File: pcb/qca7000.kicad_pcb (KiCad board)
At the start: 2 copper layers, 84.7 x 89.1 mm, 209 parts, among them J1 Conn_01x04_Pin, J10 CP/PE, J11 spare, J2 Conn_01x08_Pin, J3 CAN, J4 DEBUG, J5 UART, J6 12V_in, J7 RF, J8 CONTACTORS, J9 Temps, Q1 BC846, Q2 NCV8402xST, Q3 NCV8402xST, U1 25Q16, U2 SN65HVD234, U3 STM32F103RETx, U4 TPS54302, U5 AMS1117-3.3, U6 AMS1117-3.3, U7 74HCT04, Y1 25MHz, Y2 8MHz

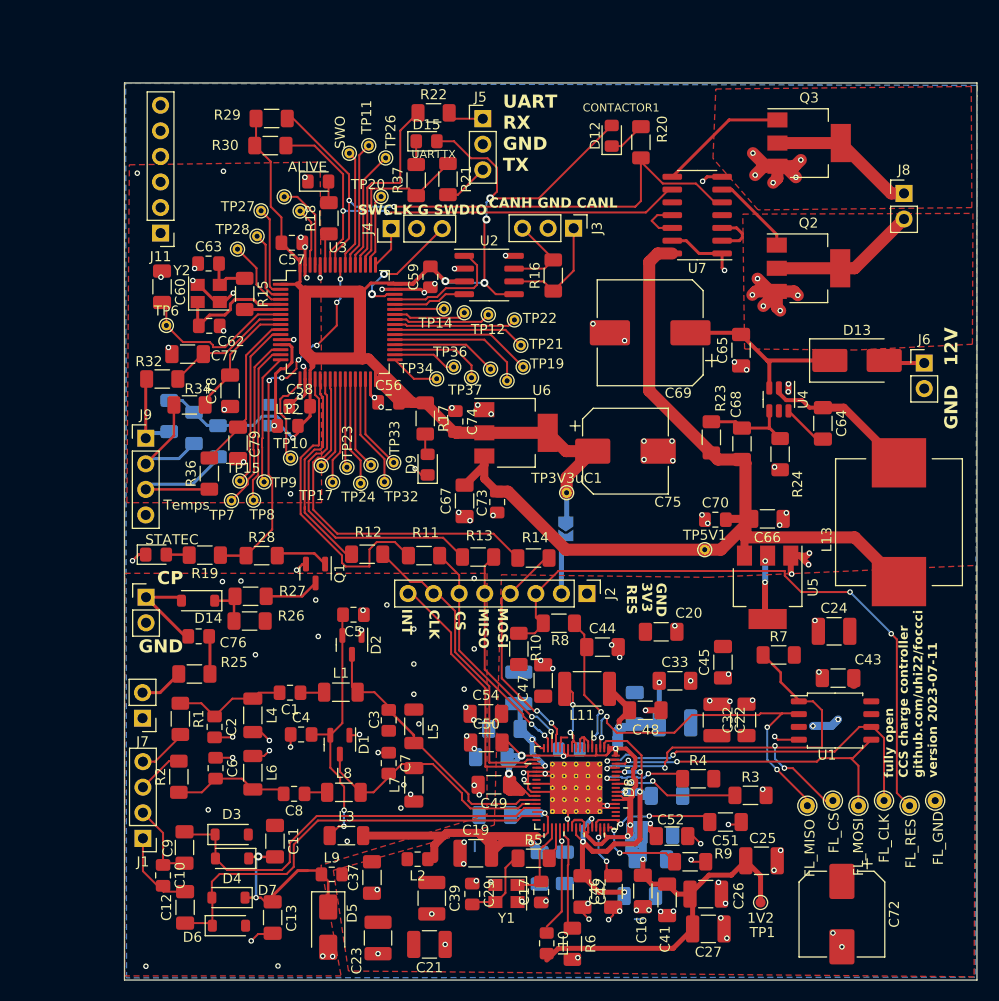
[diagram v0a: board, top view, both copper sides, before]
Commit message: fix: divider on the stepdown. fix: non-inverted contactor drivers. fix: part number of 8MHz. add: mounting holes and spare grid. add: LIM HVDC input. docu: todo list
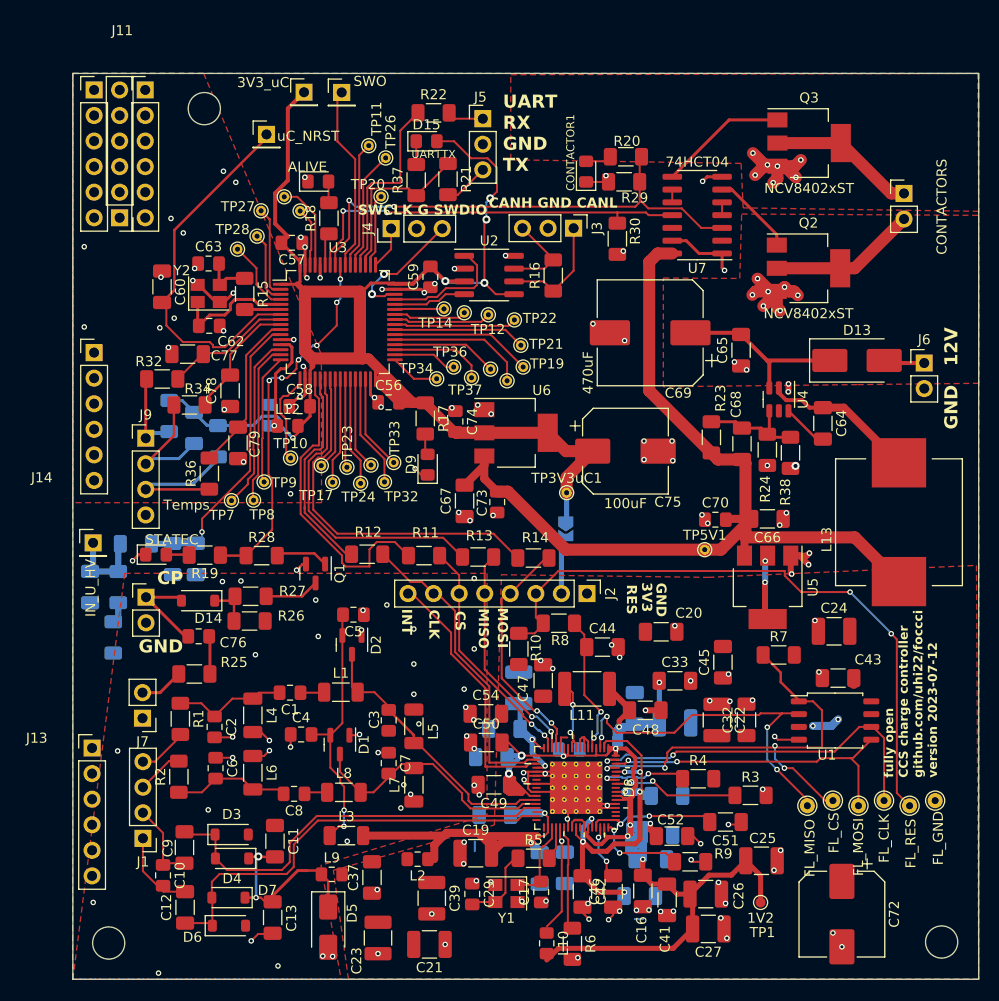
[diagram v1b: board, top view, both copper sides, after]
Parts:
- removed TP15: ~, TestPoint:TestPoint_THTPad_D1.0mm_Drill0.5mm
- removed TP35: SWO, TestPoint:TestPoint_THTPad_D1.0mm_Drill0.5mm
- removed TP6: uC_RESET, TestPoint:TestPoint_THTPad_D1.0mm_Drill0.5mm
- added C71: 100nF, Capacitor_SMD:C_1206_3216Metric_Pad1.33x1.80mm_HandSolder, B.Cu at (117.7, 90.0)
- added C80: 100nF, Capacitor_SMD:C_1206_3216Metric_Pad1.33x1.80mm_HandSolder, B.Cu at (128.2, 87.2)
- added H1: MountingHole, MountingHole:MountingHole_3.2mm_M3, F.Cu at (129.1, 42.5)
- added H2: MountingHole, MountingHole:MountingHole_3.2mm_M3, F.Cu at (119.6, 125.4)
- added H3: MountingHole, MountingHole:MountingHole_3.2mm_M3, F.Cu at (202.3, 125.3)
- added J12: spare, Connector_PinHeader_2.54mm:PinHeader_1x06_P2.54mm_Vertical, F.Cu at (123.2, 40.6)
- added J13: spare, Connector_PinHeader_2.54mm:PinHeader_1x06_P2.54mm_Vertical, F.Cu at (117.9, 106.0)
- added J14: spare, Connector_PinHeader_2.54mm:PinHeader_1x06_P2.54mm_Vertical, F.Cu at (118.1, 66.7)
- added J15: spare, Connector_PinHeader_2.54mm:PinHeader_1x06_P2.54mm_Vertical, F.Cu at (118.1, 40.6)
- added J16: uC_NRST, Connector_PinHeader_2.54mm:PinHeader_1x01_P2.54mm_Vertical, F.Cu at (135.2, 45.1)
- added J17: 3V3_uC, Connector_PinHeader_2.54mm:PinHeader_1x01_P2.54mm_Vertical, F.Cu at (139.0, 40.9)
- added J18: SWO, Connector_PinHeader_2.54mm:PinHeader_1x01_P2.54mm_Vertical, F.Cu at (142.7, 40.9)
- added J19: IN_U_HV, Connector_PinHeader_2.54mm:PinHeader_1x01_P2.54mm_Vertical, F.Cu at (118.0, 85.6)
- added R38: 22k, Resistor_SMD:R_1206_3216Metric_Pad1.30x1.75mm_HandSolder, F.Cu at (187.3, 76.7)
- added R39: 240, Resistor_SMD:R_1206_3216Metric_Pad1.30x1.75mm_HandSolder, B.Cu at (120.5, 90.0)
- added R40: 240, Resistor_SMD:R_1206_3216Metric_Pad1.30x1.75mm_HandSolder, B.Cu at (120.0, 95.0)
- added R41: 47k, Resistor_SMD:R_1206_3216Metric_Pad1.30x1.75mm_HandSolder, B.Cu at (122.3, 85.7)
- added R42: 22k, Resistor_SMD:R_1206_3216Metric_Pad1.30x1.75mm_HandSolder, B.Cu at (125.9, 87.2)
- R23: value 10k -> 100k
- R24: value 10k -> 33k
- moved R30 35.7 mm to (170.1, 55.4), turned to 90 degrees
- moved R29 35.6 mm to (170.8, 49.8)
- moved D12 4.38 mm to (167.0, 48.8)
- moved J11 4.34 mm to (120.7, 53.3)
- moved R20 2.07 mm to (170.9, 47.3), turned to 180 degrees
- moved R24 1.34 mm to (185.0, 76.4)
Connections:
- net uC_RESET renamed uC_NRST
- D12 pad 1: Net-(D12-K) -> GND
- D12 pad 2: 3V3_uC -> Net-(D12-A)
- R20 pad 2: Net-(D12-K) -> Net-(D12-A)
- R29 pad 2: 3V3_uC -> GND
- R30 pad 1: 3V3_uC -> GND
- U3 pad 11: Net-(U3-PC3) -> ADC_U_HVDC
- U7 pad 10: unconnected-(U7-Pad10) -> Net-(U7-Pad10)
- U7 pad 11: Net-(U7-Pad11) -> CONTACTOR_CONTROL2
- U7 pad 12: Net-(U7-Pad11) -> unconnected-(U7-Pad12)
- U7 pad 2: Net-(U7-Pad2) -> unconnected-(U7-Pad2)
- U7 pad 3: Net-(U7-Pad2) -> CONTACTOR_CONTROL1
- U7 pad 4: unconnected-(U7-Pad4) -> Net-(U7-Pad4)
- U7 pad 5: CONTACTOR_CONTROL1 -> Net-(U7-Pad4)
- U7 pad 9: CONTACTOR_CONTROL2 -> Net-(U7-Pad10)
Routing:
- net ADC_U_HVDC: track 0.00 -> 29.2 mm, vias 0 -> 1
- net uC_NRST: track 16.4 -> 37.4 mm
- net Net-(U3-PC3): track 16.7 -> 0.00 mm
- net CONTACTOR_CONTROL1: track 61.9 -> 50.2 mm
- net 3V3_uC: track 180.4 -> 168.8 mm
- net CONTACTOR_CONTROL2: track 50.1 -> 39.8 mm
- net Net-(J19-Pin_1): track 0.00 -> 8.60 mm
- net SWO: track 11.7 -> 18.5 mm
- net Net-(U7-Pad2): track 4.78 -> 0.00 mm
- net Net-(U7-Pad11): track 4.62 -> 0.00 mm
- net Net-(D12-K): track 3.70 -> 0.00 mm
- net Net-(D12-A): track 0.00 -> 2.60 mm
- net Net-(R39-Pad1): track 0.00 -> 2.11 mm
- net GND: track 130.8 -> 132.8 mm, vias 154 -> 169
- net Net-(U4-FB): track 9.23 -> 10.9 mm
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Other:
- board size 84.7 x 89.1 mm -> 90 x 90 mm
- board text added: "fully open CCS charge controller github.com/uhi22/foccci version 2023-07-12"
- board text removed: "fully open CCS charge controller github.com/uhi22/foccci version 2023-07-11"
